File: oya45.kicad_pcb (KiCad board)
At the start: 2 copper layers, 190.5 x 95.2 mm, 106 parts, among them U1 ProMicro

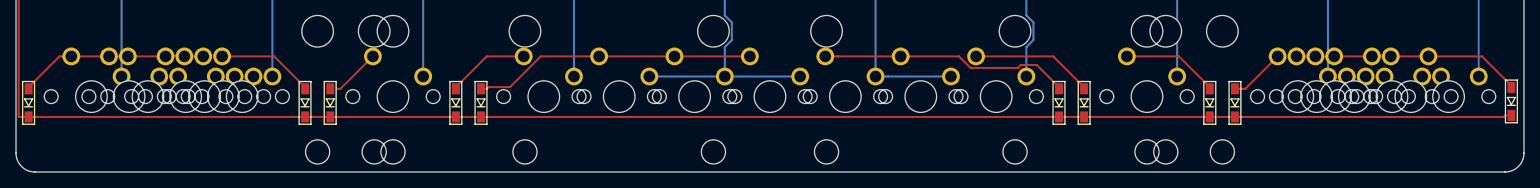
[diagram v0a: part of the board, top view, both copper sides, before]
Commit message: finished pcb
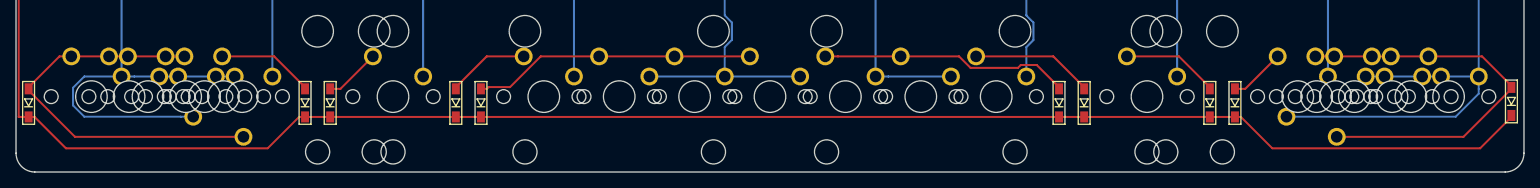
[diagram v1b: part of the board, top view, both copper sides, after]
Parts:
- turned MX51 to 0 degrees
- turned MX58 to 0 degrees
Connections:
- MX51 pad 1: Net-(MX51-Pad1) -> col0
- MX52 pad 1: Net-(MX52-Pad1) -> col0
- MX53 pad 1: Net-(MX53-Pad1) -> col0
- MX54 pad 1: Net-(MX54-Pad1) -> col0
- MX55 pad 1: Net-(MX55-Pad1) -> col0
- MX57 pad 1: Net-(MX57-Pad1) -> col9
- MX58 pad 1: Net-(MX58-Pad1) -> col9
- MX59 pad 1: Net-(MX59-Pad1) -> col9
- MX60 pad 1: Net-(MX60-Pad1) -> col9
- MX61 pad 1: Net-(MX61-Pad1) -> col9
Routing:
- net col9: track 175.0 -> 216.9 mm
- net col0: track 126.2 -> 165.2 mm
- net Net-(D31-Pad2): track 23.9 -> 51.3 mm
- net Net-(D40-Pad2): track 28.9 -> 51.3 mm
- net row4: track 324.1 -> 330.8 mm
- net Net-(D33-Pad2): track 6.30 -> 7.10 mm

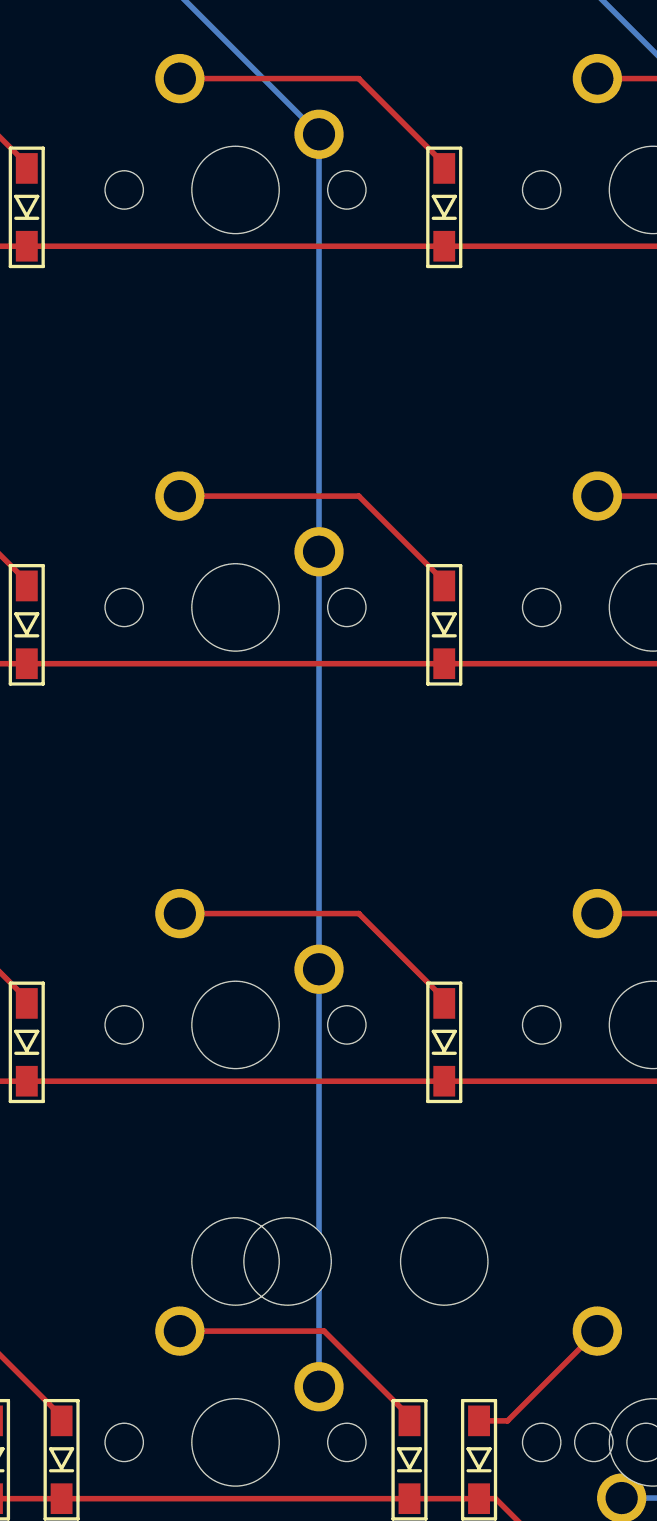
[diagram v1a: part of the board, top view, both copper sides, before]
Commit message: finished pcb
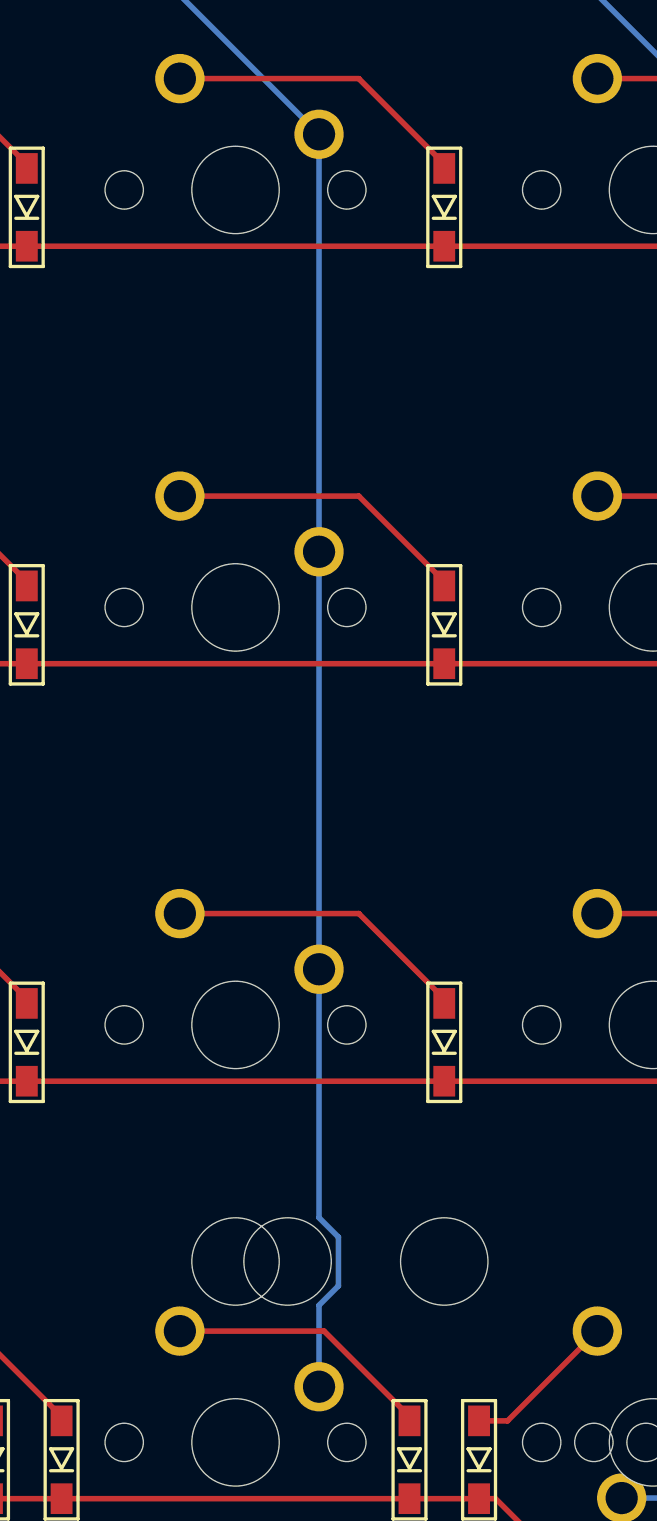
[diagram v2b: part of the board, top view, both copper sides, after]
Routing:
- net col7: track 142.6 -> 143.3 mm
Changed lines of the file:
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@@
     (thickness 1.6)
     (drawings 8)
-    (tracks 277)
+    (tracks 281)
     (zones 0)
     (modules 106)
@@
   (segment (start 84.8915 116.86875) (end 87.3125 116.86875) (width 0.254) (layer F.Cu) (net 34))
   (segment (start 84.1375 116.86875) (end 84.8915 116.86875) (width 0.254) (layer F.Cu) (net 34))
-  (segment (start 83.3835 116.86875) (end 84.1375 116.86875) (width 0.254) (layer F.Cu) (net 34))
-  (segment (start 79.420249 120.832001) (end 83.3835 116.86875) (width 0.254) (layer F.Cu) (net 34))
-  (segment (start 53.929751 120.832001) (end 79.420249 120.832001) (width 0.254) (layer F.Cu) (net 34))
-  (segment (start 49.9665 116.86875) (end 53.929751 120.832001) (width 0.254) (layer F.Cu) (net 34))
-  (segment (start 49.2125 116.86875) (end 49.9665 116.86875) (width 0.254) (layer F.Cu) (net 34))
+  (segment (start 200.8585 116.86875) (end 87.3125 116.86875) (width 0.254) (layer F.Cu) (net 34))
+  (segment (start 201.6125 116.86875) (end 200.8585 116.86875) (width 0.254) (layer F.Cu) (net 34))
   (segment (start 202.3665 116.86875) (end 201.6125 116.86875) (width 0.254) (layer F.Cu) (net 34))
   (segment (start 206.329751 120.832001) (end 202.3665 116.86875) (width 0.254) (layer F.Cu) (net 34))
   (segment (start 232.586749 120.832001) (end 206.329751 120.832001) (width 0.254) (layer F.Cu) (net 34))
-  (segment (start 236.5375 116.88125) (end 232.586749 120.832001) (width 0.254) (layer F.Cu) (net 34))
   (segment (start 236.5375 116.68125) (end 236.5375 116.88125) (width 0.254) (layer F.Cu) (net 34))
-  (segment (start 200.8585 116.86875) (end 87.3125 116.86875) (width 0.254) (layer F.Cu) (net 34))
-  (segment (start 201.6125 116.86875) (end 200.8585 116.86875) (width 0.254) (layer F.Cu) (net 34))
+  (segment (start 236.5375 116.88125) (end 232.586749 120.832001) (width 0.254) (layer F.Cu) (net 34))
+  (segment (start 49.2125 116.86875) (end 49.9665 116.86875) (width 0.254) (layer F.Cu) (net 34))
+  (segment (start 49.9665 116.86875) (end 53.929751 120.832001) (width 0.254) (layer F.Cu) (net 34))
+  (segment (start 83.3835 116.86875) (end 84.1375 116.86875) (width 0.254) (layer F.Cu) (net 34))
+  (segment (start 79.420249 120.832001) (end 83.3835 116.86875) (width 0.254) (layer F.Cu) (net 34))
+  (segment (start 53.929751 120.832001) (end 79.420249 120.832001) (width 0.254) (layer F.Cu) (net 34))
   (segment (start 49.2125 113.11875) (end 49.2125 113.31875) (width 0.254) (layer F.Cu) (net 35))
   (segment (start 53.11125 109.22) (end 49.2125 113.11875) (width 0.254) (layer F.Cu) (net 35))
@@
   (segment (start 232.82625 109.22) (end 236.5375 112.93125) (width 0.254) (layer F.Cu) (net 44))
   (segment (start 211.7725 109.22) (end 232.82625 109.22) (width 0.254) (layer F.Cu) (net 44))
+  (segment (start 214.47125 119.38) (end 230.48875 119.38) (width 0.254) (layer F.Cu) (net 44))
   (segment (start 236.5375 113.33125) (end 236.5375 113.13125) (width 0.254) (layer F.Cu) (net 44))
   (segment (start 230.48875 119.38) (end 236.5375 113.33125) (width 0.254) (layer F.Cu) (net 44))
-  (segment (start 214.47125 119.38) (end 230.48875 119.38) (width 0.254) (layer F.Cu) (net 44))
   (segment (start 128.87625 40.66875) (end 123.825 45.72) (width 0.254) (layer F.Cu) (net 45))
   (segment (start 211.1375 40.66875) (end 128.87625 40.66875) (width 0.254) (layer F.Cu) (net 45))
@@
   (segment (start 165.735 35.56) (end 160.45177 30.27677) (width 0.254) (layer B.Cu) (net 57))
   (segment (start 160.45177 30.27677) (end 134.713249 30.27677) (width 0.254) (layer B.Cu) (net 57))
-  (segment (start 194.31 54.61) (end 194.31 111.76) (width 0.254) (layer B.Cu) (net 58))
   (segment (start 184.785 45.085) (end 184.785 35.56) (width 0.254) (layer B.Cu) (net 58))
   (segment (start 194.31 54.61) (end 184.785 45.085) (width 0.254) (layer B.Cu) (net 58))
@@
   (segment (start 184.785 35.56) (end 179.04776 29.82276) (width 0.254) (layer B.Cu) (net 58))
   (segment (start 179.04776 29.82276) (end 134.525192 29.82276) (width 0.254) (layer B.Cu) (net 58))
+  (segment (start 194.31 104.045166) (end 195.195801 104.930967) (width 0.254) (layer B.Cu) (net 58))
+  (segment (start 194.31 54.61) (end 194.31 104.045166) (width 0.254) (layer B.Cu) (net 58))
+  (segment (start 195.195801 104.930967) (end 195.195801 107.159033) (width 0.254) (layer B.Cu) (net 58))
+  (segment (start 194.31 108.044834) (end 194.31 111.76) (width 0.254) (layer B.Cu) (net 58))
+  (segment (start 195.195801 107.159033) (end 194.31 108.044834) (width 0.254) (layer B.Cu) (net 58))
   (segment (start 213.36 54.61) (end 213.36 111.76) (width 0.254) (layer B.Cu) (net 59))
   (segment (start 203.835 45.085) (end 203.835 35.56) (width 0.254) (layer B.Cu) (net 59))
